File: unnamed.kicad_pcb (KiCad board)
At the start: 2 copper layers, 140 x 95 mm, 29 parts, among them J1 C128990, J2 C128990, SW1 KeySwitch, SW10 KeySwitch, SW11 KeySwitch, SW12 KeySwitch, SW13 KeySwitch, SW14 KeySwitch, SW15 KeySwitch, SW16 KeySwitch, SW17 KeySwitch, SW18 KeySwitch, SW19 KeySwitch, SW2 KeySwitch, SW20 KeySwitch, SW21 KeySwitch, SW3 KeySwitch, SW4 KeySwitch, SW5 KeySwitch, SW6 KeySwitch, SW7 KeySwitch, SW8 KeySwitch, SW9 KeySwitch, U1 Pico_SMT, U2 Pico_SMT

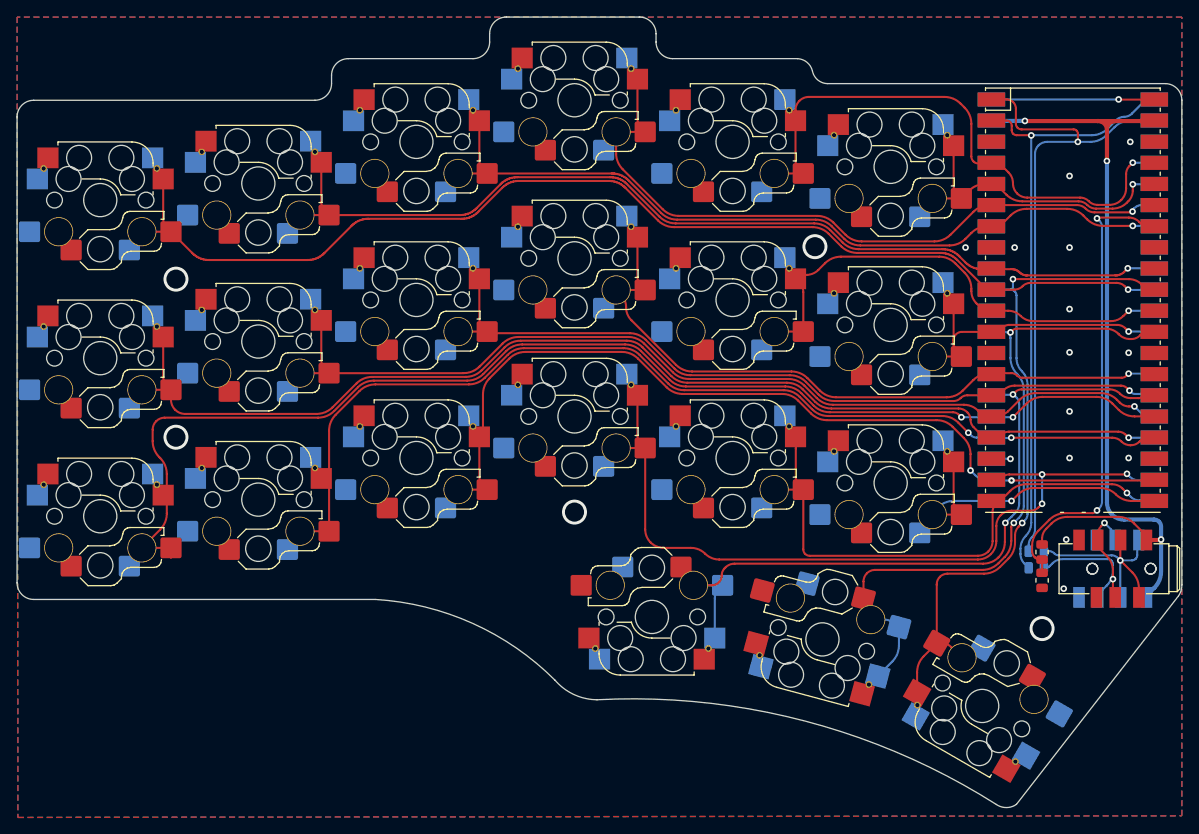
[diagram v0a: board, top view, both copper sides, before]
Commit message: update pcb and project, new 3d file for cases.
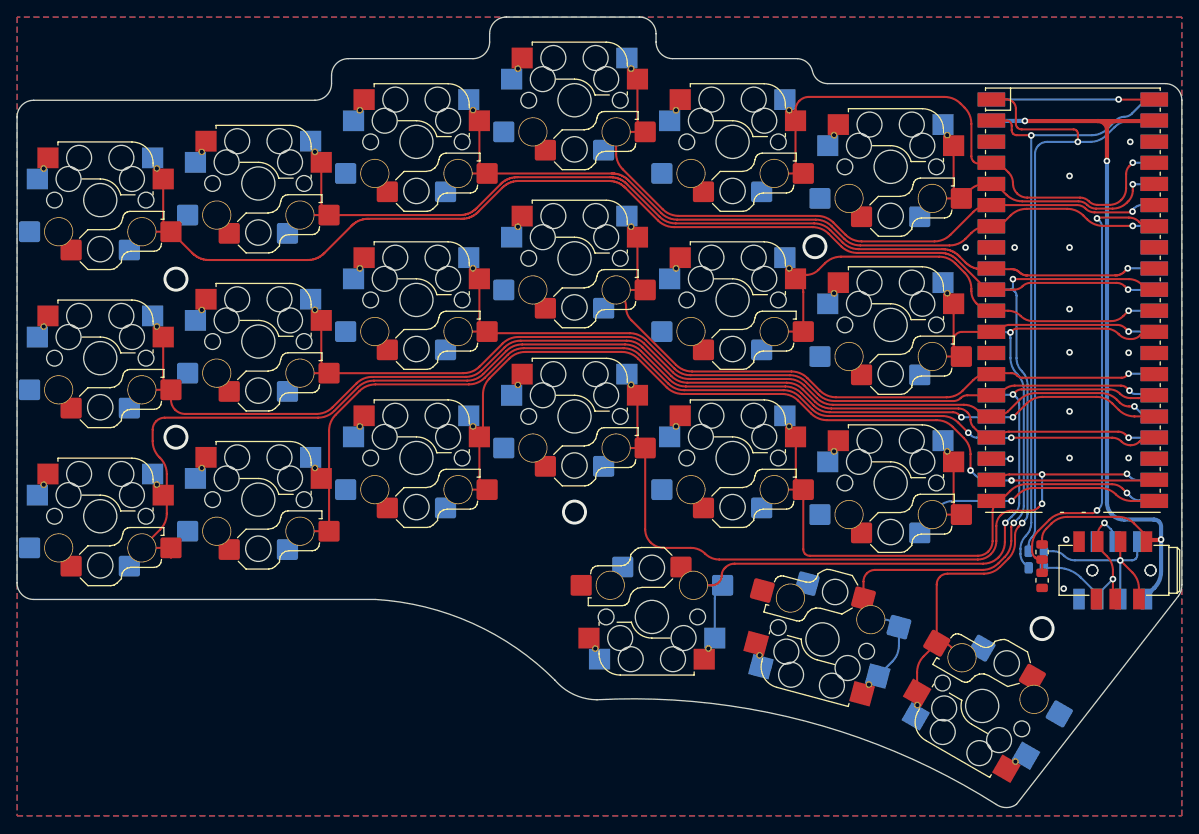
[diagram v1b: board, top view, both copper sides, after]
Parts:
- moved J1 0.19 mm to (218.4, 116.5)
- moved J2 0.19 mm to (218.4, 116.5)
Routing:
- net /U0RX: track 26.0 -> 23.3 mm
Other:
- board text added: "case cut place for TRRS connector"
- board text added: "case cut place for USB connector"
- board text added: "origin of gerber"
